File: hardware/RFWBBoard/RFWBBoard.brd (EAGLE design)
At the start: 90 x 56 mm, 95 parts, among them IC1 24LC025ST, J1 CON-71742-3003-BOT, M1 MOUNT-HOLE3.3, M2 MOUNT-HOLE3.3, M3 MOUNT-HOLE3.3, M4 MOUNT-HOLE3.3, M5 FIDUCIAL1X2, M6 FIDUCIAL1X2, M7 FIDUCIAL1X2, M8 FIDUCIAL1X2, U1 MAX2830IPC-7351, U2 LDB212G4010C-001, U3 LDB212G4010C-001, U4 AD8132MSOP8, U5 AD8132MSOP8, U6 AD8132MSOP8, U7 AD8132MSOP8, U8 LMV112, X1 SMA-SMD, X2 SMA-SMD, X3 FOX924B, X4 SMA-SMD, X5 SMA-SMD, X6 SMA-SMD, X7 SMA-SMD

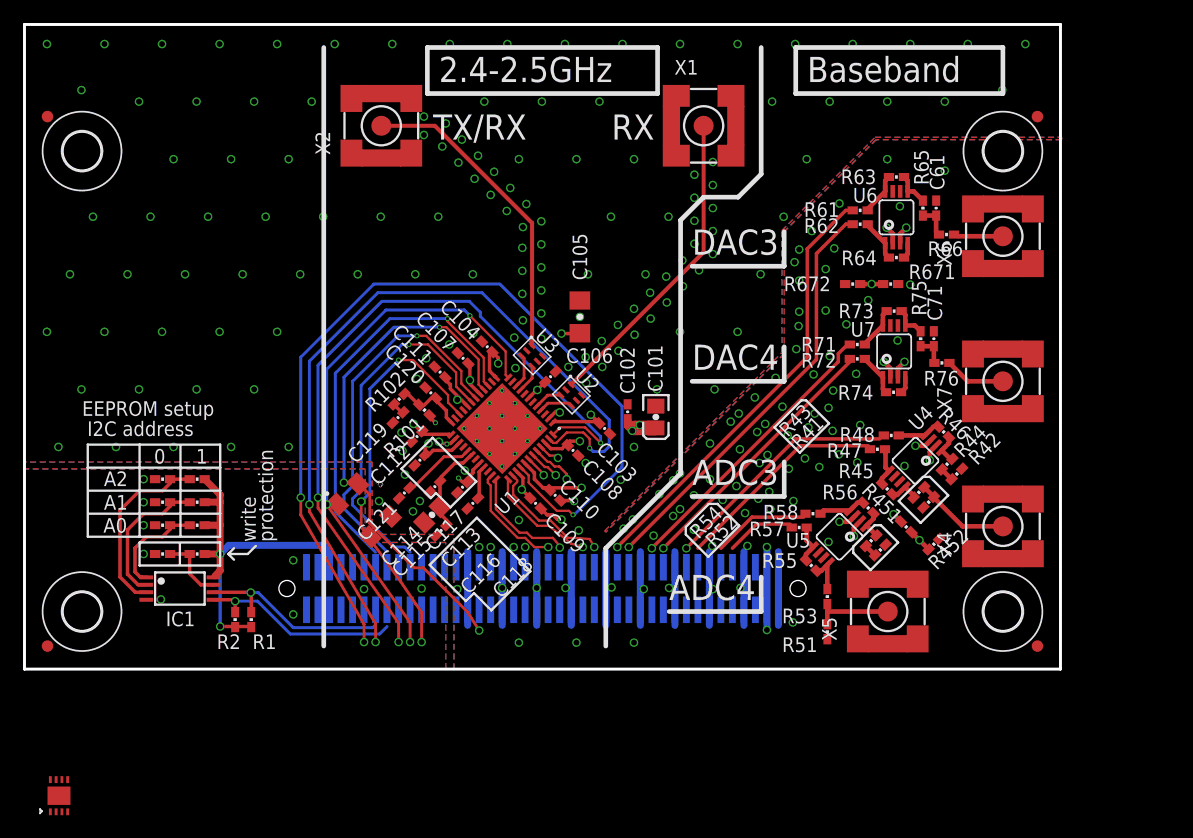
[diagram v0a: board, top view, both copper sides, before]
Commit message: - Layout update
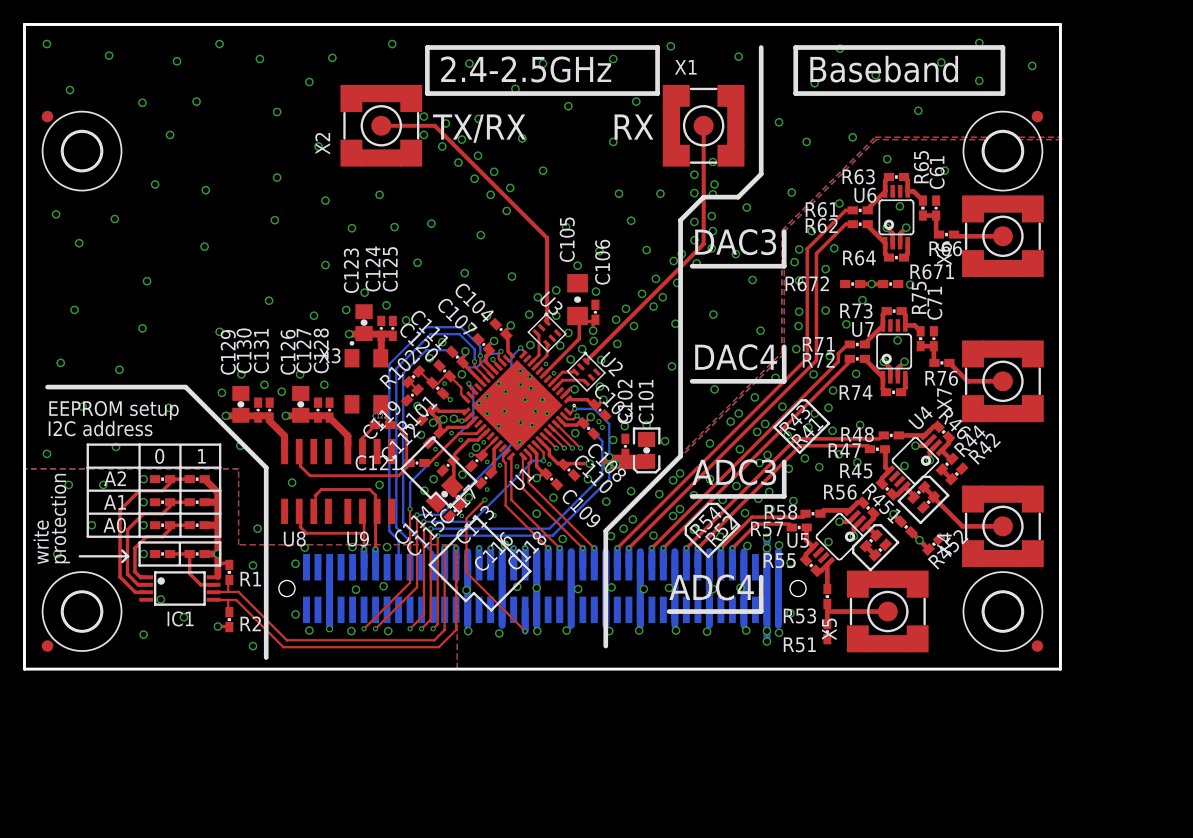
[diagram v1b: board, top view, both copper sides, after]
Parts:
- added C122: 1000pF, RFWBBoard:C0402
- added C123, C126, C129: 10uF, RFWBBoard:C0805
- added C124, C127, C130: 100nF, RFWBBoard:C0402
- added C125, C128, C131: 100pF, RFWBBoard:C0402
- added U9: ICS85320I, RFWBBoard:SOIC8
- U8: value LMV112 -> ICS83021I; device RFWBBoard:LLP-8 -> RFWBBoard:SOIC8
- moved LOGO3 55.9 mm to (47.5, 60.5)
- moved LOGO1 37.8 mm to (32.5, 61.0)
- moved U8 34.7 mm to (24.5, 16.3)
- moved LOGO2 20.8 mm to (17.5, 60.5)
- moved X3 11.2 mm to (29.7, 25.0), turned to 270 degrees
- moved C106 6.82 mm to (49.6, 31.0), turned to 270 degrees
- moved R1 4.52 mm to (17.8, 8.40), turned to 90 degrees
- moved C101 3.01 mm to (54.0, 19.0)
- moved C102 3.01 mm to (52.2, 19.4)
- moved C121 2.82 mm to (34.1, 17.9), turned to 180 degrees
- moved C118 2.62 mm to (39.3, 18.1)
- moved C109 2.52 mm to (45.8, 16.5)
- moved C110 2.51 mm to (47.3, 17.3)
- moved C117 2.48 mm to (40.1, 16.6)
- moved U1 2.39 mm to (42.8, 22.9)
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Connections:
- removed net GND: U8.5
- removed net VCC: U8.1
- new net N$37: J1.11
- new net N$38: J1.13
- new net N$39: C122.1, U9.7
- new net N$40: J1.23
- new net N$41: J1.19
- new net N$42: J1.21
- net !SHDN: no longer J1.19
- net A3V3: now also C123.1, C124.1, C125.1, C126.1, C127.1, C128.1, C129.1, C130.1, C131.1, U8.8, U9.8
- net AGND: now also C123.2, C124.2, C125.2, C126.2, C127.2, C128.2, C129.2, C130.2, C131.2, U8.5, U9.5
- net ANTSEL: no longer J1.13
- net CLK1: now also U8.2, U9.2
- net CLK2: now also U8.3, U9.3
- net LD: no longer J1.21
- net N$36: now also C122.2, U8.7
- net RXHP: no longer J1.11
- net RXTX: no longer J1.17
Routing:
- net A3V3: track 181.8 -> 83.2 mm, vias 21 -> 27
- net RXHP: track 79.1 -> 24.1 mm
- net ANTSEL: track 68.5 -> 33.0 mm
- net RXTX: track 63.7 -> 34.1 mm
- net RSSI: track 45.4 -> 29.0 mm
- net !SHDN: track 47.6 -> 31.4 mm
- net N$36: track 0.00 -> 15.6 mm
- net I2C_SDA: track 17.5 -> 31.6 mm
- net I2C_SCL: track 17.2 -> 30.4 mm
- net CLK2: track 0.00 -> 12.1 mm, vias 0 -> 1
- net CLK1: track 0.00 -> 10.4 mm, vias 0 -> 1
- net LD: track 34.9 -> 26.0 mm
- net !CS: track 36.0 -> 28.3 mm
- net TXBBQ-: track 10.9 -> 14.4 mm
- net AGND: track 69.6 -> 66.1 mm, vias 244 -> 293
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
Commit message: - Decoupling capacitors - Layout update - Schematic update
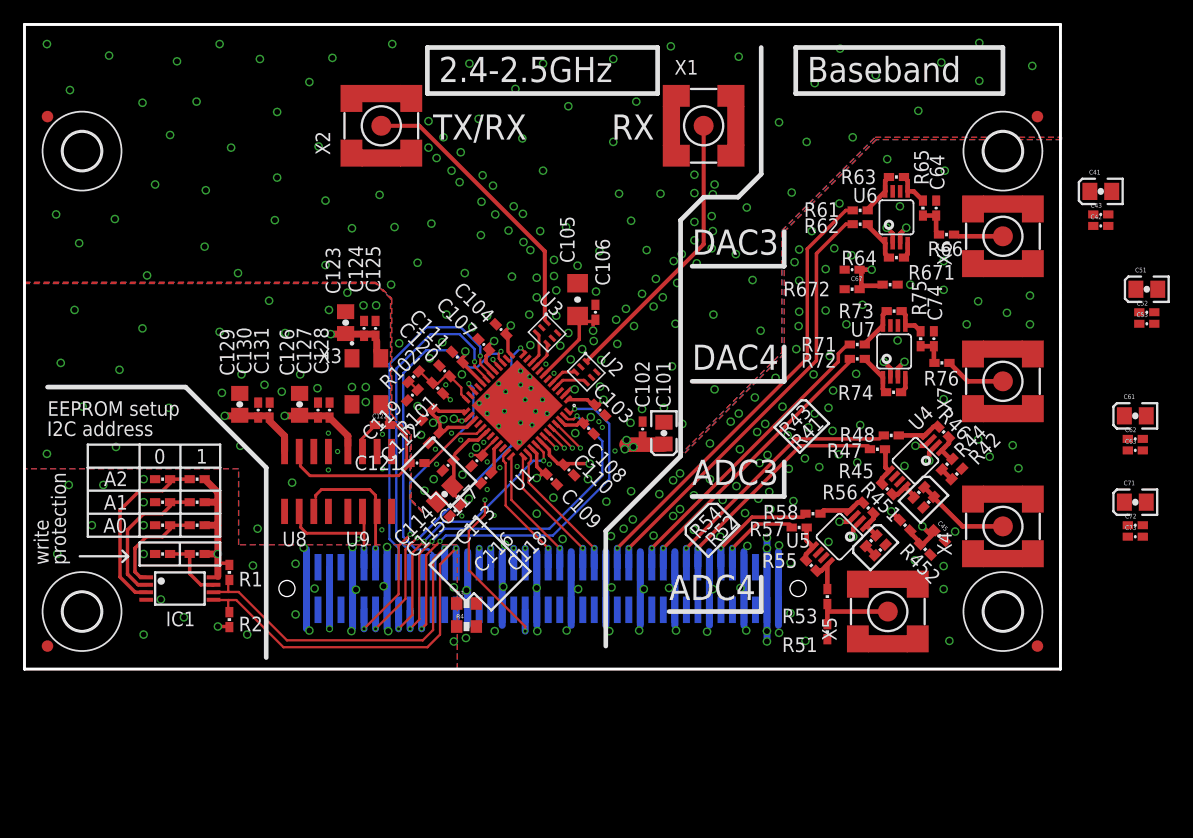
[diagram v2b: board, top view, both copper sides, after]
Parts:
- added C41, C51: 10uF, RFWBBoard:CPOL2012
- added C42, C45, C52, C62, C67, C72: 100nF, RFWBBoard:C0402
- added C43, C53, C63, C73: 10nF, RFWBBoard:C0402
- added C64, C74: 100pF, RFWBBoard:C0402
- added R3, R4: DNP, RFWBBoard:R0603
- C61, C71: value 100pF -> 10uF; device RFWBBoard:C0402 -> RFWBBoard:CPOL2012
- RA00, RA01, RA10, RA11, RA20, RA21, RWP0, RWP1: value NONE -> DNP
- moved C61 25.0 mm to (96.5, 22.0), turned to 0 degrees
- moved C71 22.5 mm to (96.5, 14.5), turned to 0 degrees
- moved C101 2.12 mm to (55.5, 20.5)
- moved C102 2.12 mm to (53.7, 20.9)
- moved C123 1.60 mm to (27.9, 30.1)
- moved C124 1.50 mm to (29.5, 29.6)
- moved C125 1.50 mm to (30.5, 29.6)
- moved R452 0.87 mm to (78.2, 10.4), turned to 135 degrees
- moved R672 0.45 mm to (71.9, 33.0)
- moved R451 0.18 mm to (76.5, 12.5)
- moved C126 0.10 mm to (23.9, 23.0)
- moved C129 0.10 mm to (18.7, 23.0)
- moved R671 0.07 mm to (75.2, 33.4)
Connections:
- removed net N$37: J1.11
- removed net N$38: J1.13
- removed net N$40: J1.23
- removed net N$41: J1.19
- removed net N$42: J1.21
- net !SHDN: now also J1.13
- net A3V3: now also C41.+, C42.1, C43.1, C51.+, C52.1, C53.1, C61.+, C62.1, C63.1, C71.+, C72.1, C73.1
- net AGND: now also C41.-, C42.2, C43.2, C45.2, C51.-, C52.2, C53.2, C61.-, C62.2, C63.2, C64.2, C67.2, C71.-, C72.2, C73.2, C74.2, R3.2, R4.2; no longer C61.2, C71.2
- net ANTSEL: now also J1.19
- net DGND: now also R3.1, R4.1
- net LD: now also J1.11
- net N$27: now also C64.1; no longer C61.1
- net N$33: now also C74.1; no longer C71.1
- net RXHP: now also J1.17
- net RXTX: now also J1.21
- net V_BIAS_ADC: now also C45.1
- net V_BIAS_DAC: now also C67.1
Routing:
- net DGND: track 0.00 -> 20.7 mm, vias 23 -> 26
- net V_BIAS_DAC: track 17.7 -> 19.8 mm
- net RXTX: track 34.1 -> 35.8 mm
- net LD: track 26.0 -> 27.7 mm
- net ANTSEL: track 33.0 -> 34.4 mm
- net A3V3: track 83.2 -> 82.2 mm
- net RXHP: track 24.1 -> 25.2 mm
- net !CS: track 28.3 -> 29.1 mm
- net V_BIAS_ADC: track 17.9 -> 18.6 mm
- net N$9: track 25.2 -> 24.6 mm
- net I2C_SDA: track 31.6 -> 31.0 mm
- net I2C_SCL: track 30.4 -> 29.8 mm
- net !SHDN: track 31.4 -> 32.0 mm
- net AGND: vias 293 -> 334
- added copper zone on layer 1, net N$43
- added copper zone on layer 14, net N$43
- added copper zone on layer 15, net N$43
- added copper zone on layer 16, net N$43
- added copper zone on layer 2, net N$43
- added copper zone on layer 3, net N$43

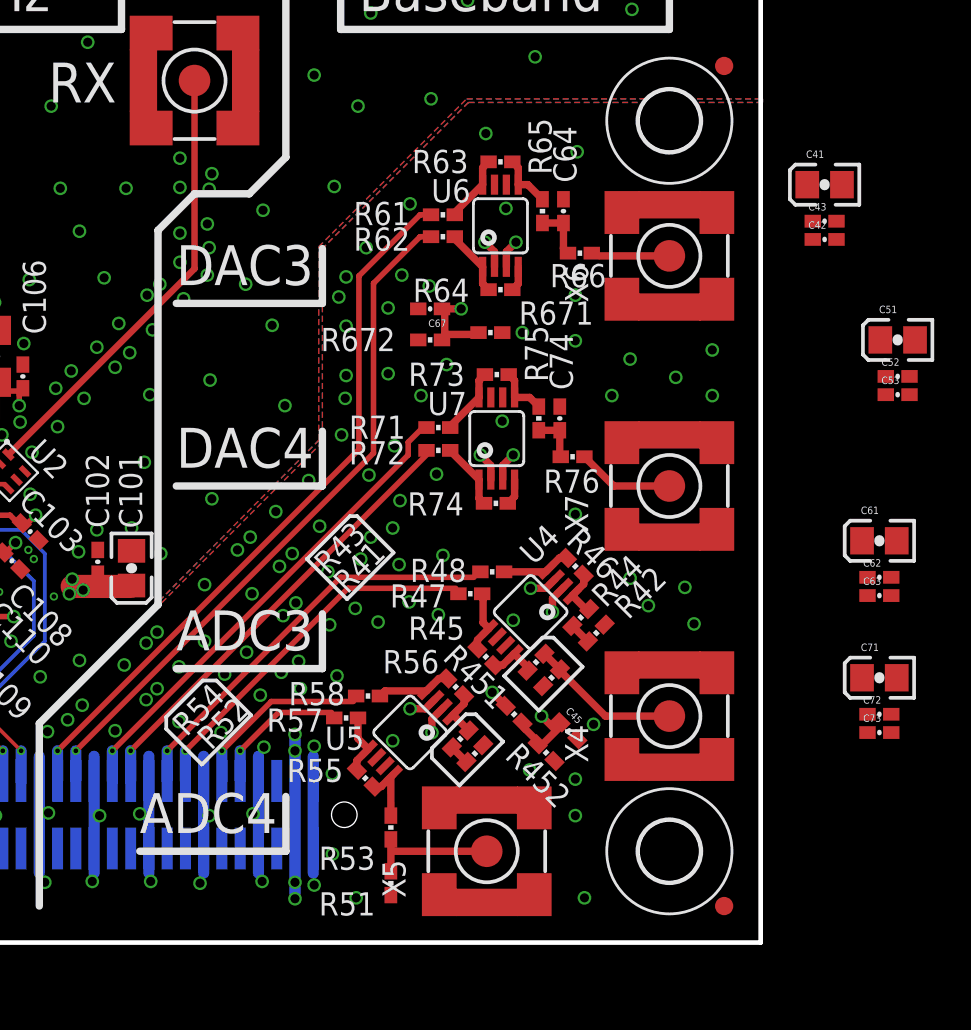
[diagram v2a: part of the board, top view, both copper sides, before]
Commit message: - Layout update
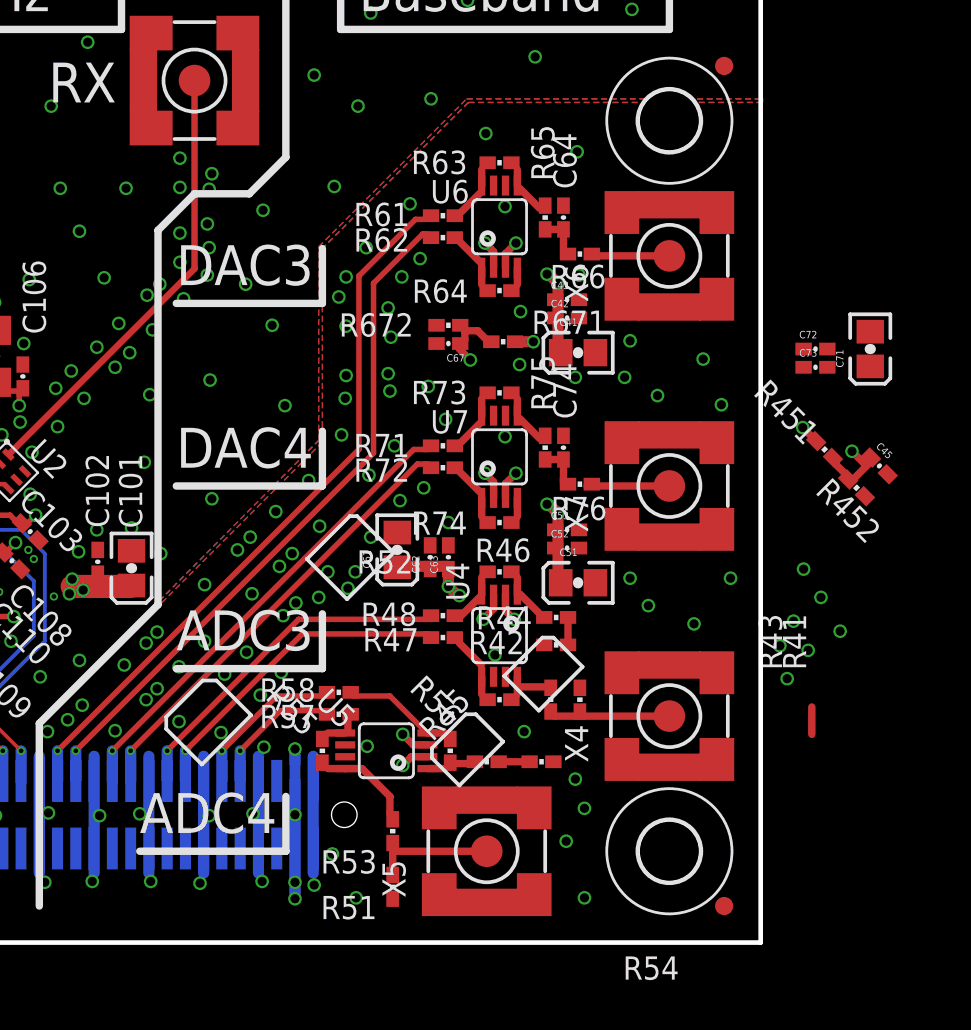
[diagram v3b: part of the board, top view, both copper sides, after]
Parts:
- moved C61 26.4 mm to (70.1, 21.5), turned to 90 degrees
- moved C62 24.6 mm to (71.9, 21.1), turned to 90 degrees
- moved C63 23.7 mm to (72.9, 21.1), turned to 90 degrees
- moved C45 22.3 mm to (96.5, 26.1)
- moved R451 22.3 mm to (93.5, 27.0)
- moved R452 22.3 mm to (95.2, 24.9)
- moved C51 22.0 mm to (80.0, 19.7)
- moved C52 20.4 mm to (79.4, 21.6)
- moved C72 20.3 mm to (93.0, 32.5)
- moved C73 20.3 mm to (93.0, 31.5)
- moved C53 19.6 mm to (79.4, 22.6)
- moved C71 18.0 mm to (96.0, 32.5), turned to 90 degrees
- moved C41 16.3 mm to (80.0, 32.3)
- moved C42 14.7 mm to (79.4, 34.2)
- moved C43 14.7 mm to (79.4, 35.2)
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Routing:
- net A3V3: track 82.2 -> 94.6 mm, vias 27 -> 33
- net ADC3-: track 22.4 -> 19.1 mm
- net ADC3+: track 20.1 -> 17.6 mm
- net V_BIAS_ADC: track 18.6 -> 16.8 mm
- net N$18: track 3.34 -> 1.65 mm
- net N$20: track 3.35 -> 5.03 mm
- net N$19: track 4.09 -> 5.64 mm
- net ADC4-: track 9.97 -> 8.69 mm
- net N$13: track 3.76 -> 2.65 mm
- net N$23: track 3.67 -> 2.57 mm
- net N$28: track 3.69 -> 2.62 mm
- net N$24: track 3.67 -> 2.70 mm
- net N$30: track 3.67 -> 2.72 mm
- net N$21: track 2.61 -> 1.75 mm
- net N$27: track 2.90 -> 2.05 mm
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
